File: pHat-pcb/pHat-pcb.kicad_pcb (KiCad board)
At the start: 2 copper layers, 65 x 30 mm, 16 parts, among them J1 Conn_02x20_Odd_Even, J2 Conn_01x24_Male, J3 Conn_Active_High, J4 Conn_Bat, J5 Conn_I2C, J8 Conn_Active_Low, SW1 SW_Push, U1 TPS61023_Breakout, U2 74HCT74, U3 DS3231M, U4 74HC03

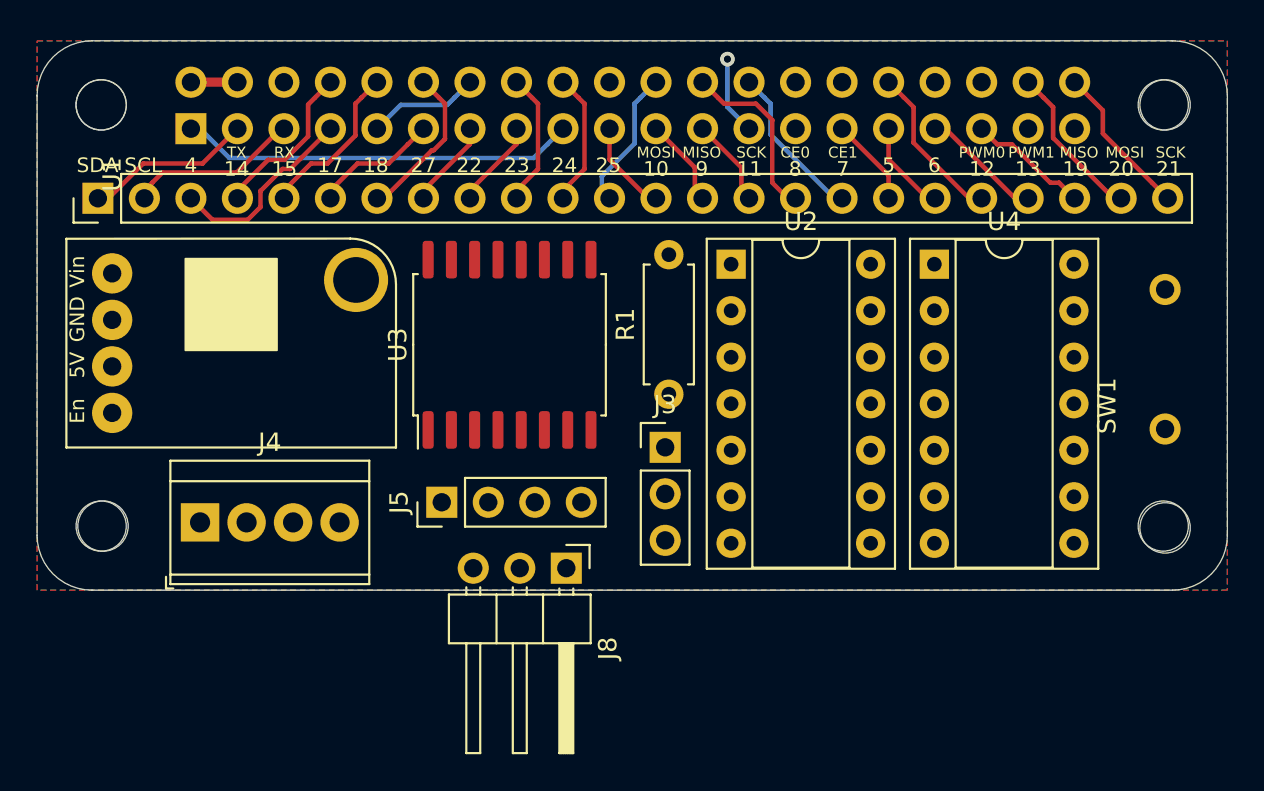
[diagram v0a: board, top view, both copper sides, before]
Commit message: Rev 1: layout complete
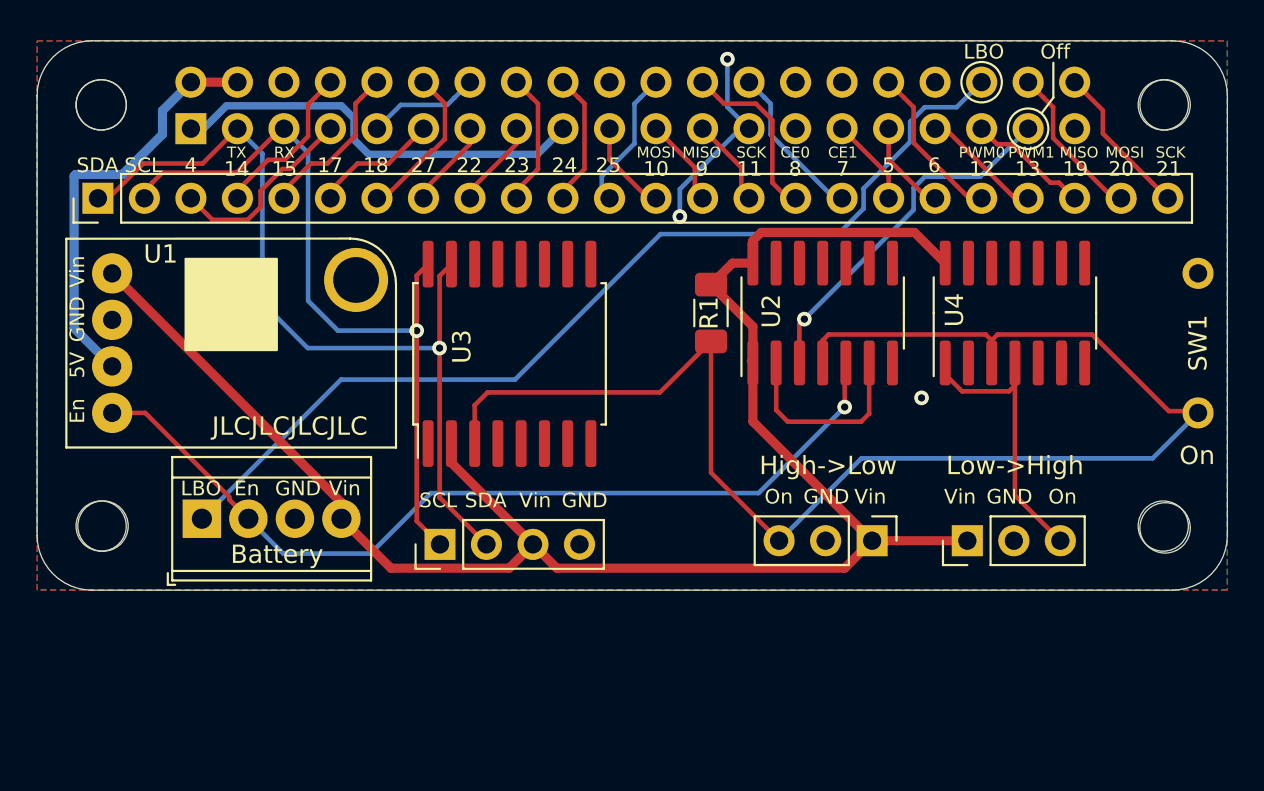
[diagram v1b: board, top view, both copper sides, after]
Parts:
- J8: footprint Connector_PinHeader_2.54mm:PinHeader_1x03_P2.54mm_Horizontal -> Connector_PinHeader_2.54mm:PinHeader_1x03_P2.54mm_Vertical
- R1: footprint Resistor_THT:R_Axial_DIN0207_L6.3mm_D2.5mm_P7.62mm_Horizontal -> Resistor_SMD:R_1206_3216Metric_Pad1.30x1.75mm_HandSolder
- U2, U4: footprint Package_DIP:DIP-14_W7.62mm_Socket -> user:SO-14_3.9x8.65mm_P1.27mm_HandSolder
- U3: footprint Package_SO:SOIC-16W_7.5x10.3mm_P1.27mm -> user:SOIC-16W_7.5x10.3mm_P1.27mm_HandSolder
- moved J3 17.3 mm to (100.8, 76.3), turned to 90 degrees
- moved J8 16.8 mm to (95.6, 76.3)
- moved SW1 8.69 mm to (113.4, 61.7), turned to 270 degrees
- moved U2 5.67 mm to (92.9, 63.9), turned to 90 degrees
- moved U4 5.14 mm to (103.4, 63.9), turned to 90 degrees
- moved R1 5.00 mm to (86.8, 63.9)
- moved J5 2.30 mm to (72.0, 76.5)
- moved U3 0.50 mm to (75.8, 66.1)
- moved J4 0.22 mm to (59.0, 75.1)
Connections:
- J4 pad 3: Net-(J4-Pad3) -> GND
- J4 pad 4: Net-(J4-Pad4) -> /Vin
- J5 pad 1: Net-(J5-Pad1) -> /GPIO3(SCL1)
- J5 pad 2: Net-(J5-Pad2) -> /GPIO2(SDA1)
- J8 pad 1: GND -> /Vin
- J8 pad 2: /Vin -> GND
- U1 pad 1: Net-(J4-Pad4) -> /Vin
- U1 pad 2: Net-(J4-Pad3) -> GND
- U3 pad 15: Net-(J5-Pad2) -> /GPIO2(SDA1)
- U3 pad 16: Net-(J5-Pad1) -> /GPIO3(SCL1)
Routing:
- net /Vin: track 0.00 -> 96.1 mm
- net /1~PRE: track 0.00 -> 79.8 mm
- net /GPIO16: track 0.00 -> 53.7 mm
- net /En: track 0.00 -> 49.0 mm, vias 0 -> 1
- net /GPIO2(SDA1): track 9.19 -> 46.6 mm, vias 0 -> 1
- net /GPIO3(SCL1): track 9.61 -> 42.3 mm, vias 0 -> 1
- net +5V: track 2.54 -> 23.1 mm
- net /GPIO26: track 0.00 -> 20.1 mm, vias 0 -> 1
- net Net-(J3-Pad3): track 0.00 -> 16.9 mm
- net Net-(U2-Pad2): track 0.00 -> 10.9 mm
- net GND: track 10.4 -> 17.1 mm, vias 1 -> 3
- net +3V3: track 21.6 -> 23.2 mm
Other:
- net class +3,3V added: clearance 0.2, trace_width 0.4, via_dia 0.8, via_drill 0.4
- rule pad_to_mask_clearance: 0.051 -> 0
- board text added: "Battery"
- board text added: "En"
- board text added: "GND"
- board text added: "High->Low"
- board text added: "JLCJLCJLCJLC"
- board text added: "LBO"
- board text added: "Low->High"
- board text added: "Off"
- board text added: "On"
- board text added: "Rev 1"
- board text added: "Vin"
- board text added: "https://github.com/bablokb/pcb-pi-batman"
